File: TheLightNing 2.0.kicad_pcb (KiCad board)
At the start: 2 copper layers, 71 x 51 mm, 27 parts, among them J1 motores izq, J2 motores der, J3 batt, J4 LED_izq, SW1 SW_SPDT, U1 L298(H)N, U2 ESP32_DEVKITC, U3 L7805

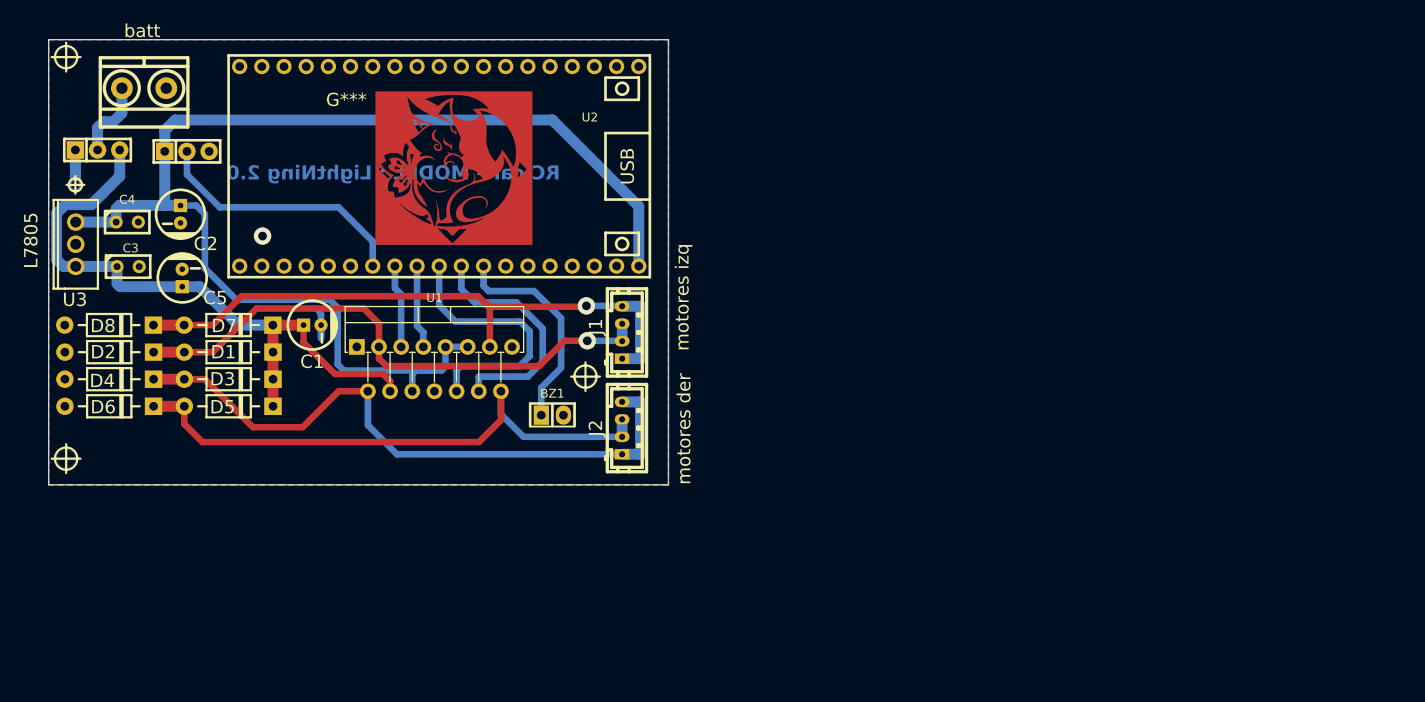
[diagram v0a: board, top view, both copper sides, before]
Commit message: re-made
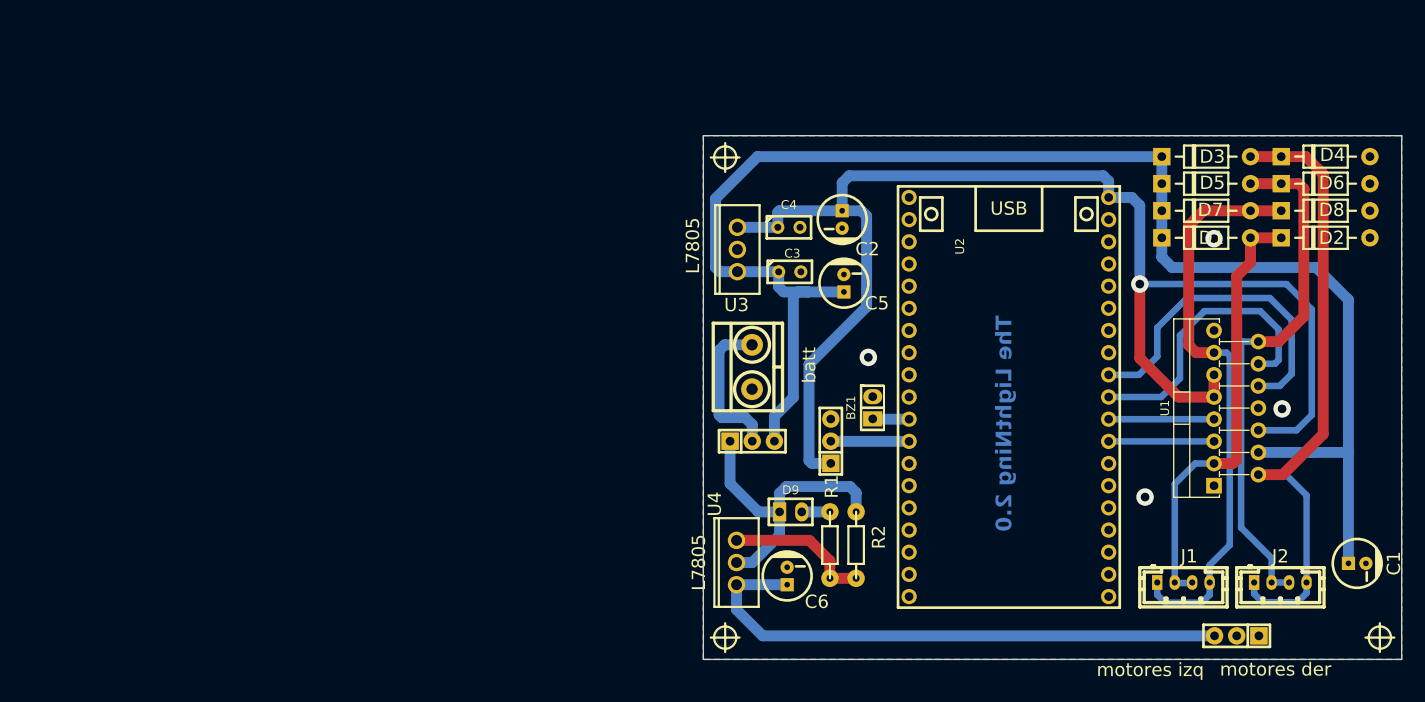
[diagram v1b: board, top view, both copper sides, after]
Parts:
- removed G***: LOGO, logo:yae
- removed H1: salida, EESTN5:hole_1mm
- removed the hole_2mm at (96.5, 67.6)
- removed the hole_2mm at (37.0, 77.0)
- removed the hole_2mm at (37.0, 31.0)
- added C6: 100uF 25v, EESTN5:CAP_ELEC_5x11mm, F.Cu at (119.6, 90.4)
- added D9: LED, EESTN5:Pin_strip_2, F.Cu at (120.0, 83.1)
- added J5: dc jack, EESTN5:Pin_Strip_3, F.Cu at (171.1, 97.3)
- added R1: 330, EESTN5:RES0.3, F.Cu at (124.5, 86.9)
- added R2: 22 2W, EESTN5:RES0.3, F.Cu at (127.5, 86.9)
- added U4: L7805, EESTN5:TO-220, F.Cu at (113.8, 88.9)
- added hole_2mm: VAL**, EESTN5:hole_2mm, F.Cu at (187.5, 97.5)
- added hole_2mm: VAL**, EESTN5:hole_2mm, F.Cu at (112.5, 97.5)
- added hole_2mm: VAL**, EESTN5:hole_2mm, F.Cu at (112.5, 42.5)
- moved D4 141.7 mm to (181.3, 42.4), turned to 180 degrees
- moved D6 141.7 mm to (181.3, 45.5), turned to 180 degrees
- moved D8 140.0 mm to (181.3, 48.6), turned to 180 degrees
- moved D2 140.0 mm to (181.3, 51.7), turned to 180 degrees
- moved C1 122.8 mm to (184.9, 89.0)
- moved D3 114.8 mm to (167.6, 42.4), turned to 180 degrees
- moved D5 114.8 mm to (167.6, 45.5), turned to 180 degrees
- moved D7 112.8 mm to (167.6, 48.6), turned to 180 degrees
- moved D1 112.7 mm to (167.6, 51.7), turned to 180 degrees
- moved U1 99.5 mm to (168.5, 80.1), turned to 90 degrees
- moved SW1 82.1 mm to (115.6, 75.0)
- moved J4 80.9 mm to (124.6, 75.0), turned to 90 degrees
- moved J2 77.5 mm to (176.1, 91.2), turned to 0 degrees
- moved J3 76.6 mm to (115.6, 66.5), turned to 90 degrees
- moved C3 75.8 mm to (119.9, 55.6)
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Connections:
- SW1 pad 1: Net-(SW1-A) -> /Cargador
- U2 pad 10: /IN3 -> /IN4
- U2 pad 11: /IN4 -> /IN3
- U2 pad 12: /buzz -> unconnected-(U2-IO14-Pad12)
- U2 pad 30: unconnected-(U2-IO18-Pad30) -> /buzz
- U2 pad 31: unconnected-(U2-IO19-Pad31) -> /led
- U2 pad 7: /led -> unconnected-(U2-IO32-Pad7)
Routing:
- net VCC: track 74.1 -> 172.8 mm
- net Net-(J5-P3): track 0.00 -> 64.7 mm
- net /Cargador: track 0.00 -> 34.5 mm
- net /led: track 29.9 -> 8.98 mm
- net /buzz: track 24.7 -> 4.19 mm
- net +5V: track 143.3 -> 160.7 mm, vias 0 -> 1
- net Net-(U4-OUT): track 0.00 -> 16.7 mm
- net Net-(D1-A): track 64.0 -> 51.1 mm, vias 1 -> 0
- net Net-(SW1-B): track 8.88 -> 17.6 mm
- net /IN3: track 30.4 -> 38.2 mm
- net Net-(D5-A): track 66.6 -> 60.3 mm
- net /IN4: track 27.3 -> 33.3 mm
- net GND: track 4.58 -> 0.00 mm, vias 1 -> 4
- net Net-(SW1-A): track 4.00 -> 0.00 mm
- net Net-(D7-A): track 70.4 -> 66.6 mm, vias 1 -> 0
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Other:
- board size 71 x 51 mm -> 80 x 60 mm
- board text added: "The LightNing 2.0"
- board text removed: "RC car - MODEL : LightNing 2.0"
